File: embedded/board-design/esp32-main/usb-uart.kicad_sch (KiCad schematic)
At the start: 16 parts, among them J4 0473460001, U3 FT231XS

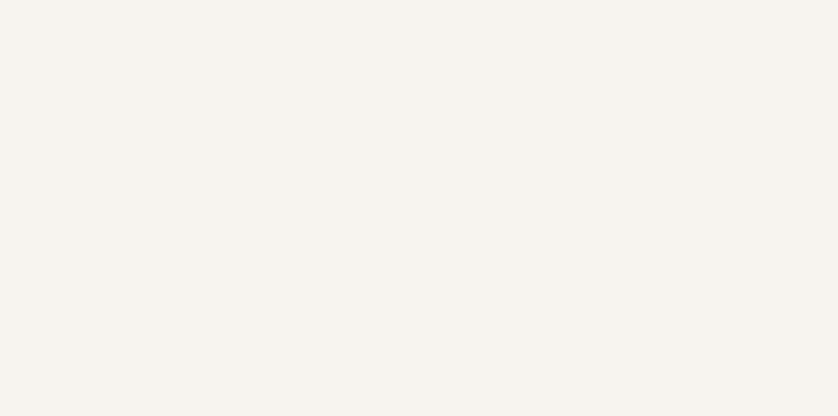
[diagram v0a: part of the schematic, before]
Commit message: [bike-embedded-app]
Signed-off-by: Nicolae-Andrei Vasile <vasilenicolaeandrei@gmail.com>
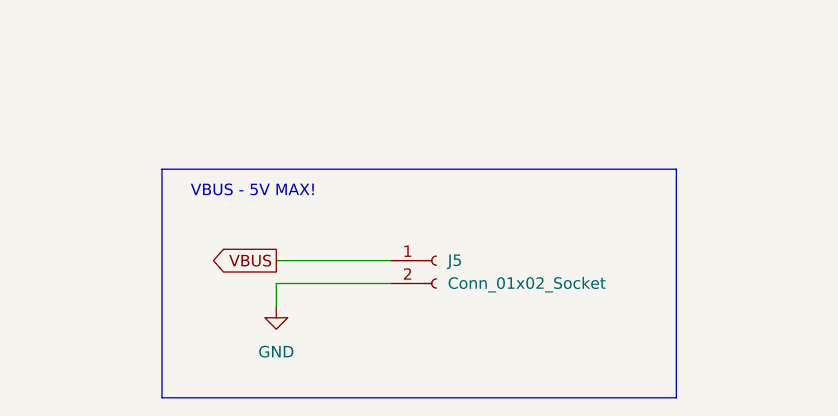
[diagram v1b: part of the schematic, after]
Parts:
- added J5: Conn_01x02_Socket, Connector_PinHeader_1.27mm:PinHeader_1x02_P1.27mm_Vertical, symbol Connector:Conn_01x02_Socket
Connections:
- net GND: now also J5.2 (Pin_2)
- net VBUS: now also J5.1 (Pin_1)
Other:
- note added: "VBUS - 5V MAX!"
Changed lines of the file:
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@@
 	(wire
 		(pts
+			(xy 127 176.53) (xy 139.7 176.53)
+		)
+		(stroke
+			(width 0)
+			(type default)
+		)
+	)
+	(wire
+		(pts
 			(xy 148.59 60.96) (xy 148.59 63.5)
 		)
@@
 	(wire
 		(pts
+			(xy 127 179.07) (xy 127 181.61)
+		)
+		(stroke
+			(width 0)
+			(type default)
+		)
+	)
+	(wire
+		(pts
 			(xy 118.11 86.36) (xy 147.32 86.36)
 		)
@@
 		)
 	)
+	(polyline
+		(pts
+			(xy 114.3 191.77) (xy 171.45 191.77)
+		)
+		(stroke
+			(width 0)
+			(type default)
+		)
+	)
 	(wire
 		(pts
@@
 		)
 	)
+	(polyline
+		(pts
+			(xy 171.45 166.37) (xy 114.3 166.37)
+		)
+		(stroke
+			(width 0)
+			(type default)
+		)
+	)
 	(wire
 		(pts
@@
 	(wire
 		(pts
+			(xy 139.7 179.07) (xy 127 179.07)
+		)
+		(stroke
+			(width 0)
+			(type default)
+		)
+	)
+	(wire
+		(pts
 			(xy 68.58 111.76) (xy 68.58 129.54)
 		)
@@
 		)
 	)
+	(polyline
+		(pts
+			(xy 171.45 191.77) (xy 171.45 166.37)
+		)
+		(stroke
+			(width 0)
+			(type default)
+		)
+	)
 	(wire
 		(pts
@@
 		)
 	)
+	(polyline
+		(pts
+			(xy 114.3 166.37) (xy 114.3 191.77)
+		)
+		(stroke
+			(width 0)
+			(type default)
+		)
+	)
 	(wire
 		(pts
@@
 		)
 	)
+	(text "VBUS - 5V MAX!"
+		(exclude_from_sim no)
+		(at 124.46 168.91 0)
+		(effects
+			(font
+				(size 1.27 1.27)
+			)
+		)
+	)
 	(label "D+"
 		(at 78.74 96.52 0)
@@
 	)
 	(global_label "VBUS"
+		(shape output)
+		(at 127 176.53 180)
+		(fields_autoplaced yes)
+		(effects
+			(font
+				(size 1.27 1.27)
+			)
+			(justify right)
+		)
+		(property "Intersheetrefs" "${INTERSHEET_REFS}"
+			(at 119.1162 176.53 0)
+			(effects
+				(font
+					(size 1.27 1.27)
+				)
+				(justify right)
+				(hide yes)
+			)
+		)
+	)
+	(global_label "VBUS"
 		(shape input)
 		(at 236.22 113.03 0)
@@
 	)
 	(symbol
+		(lib_id "Connector:Conn_01x02_Socket")
+		(at 144.78 176.53 0)
+		(unit 1)
+		(exclude_from_sim no)
+		(in_bom yes)
+		(on_board yes)
+		(dnp no)
+		(fields_autoplaced yes)
+		(property "Reference" "J5"
+			(at 146.05 176.5299 0)
+			(effects
+				(font
+					(size 1.27 1.27)
+				)
+				(justify left)
+			)
+		)
+		(property "Value" "Conn_01x02_Socket"
+			(at 146.05 179.0699 0)
+			(effects
+				(font
+					(size 1.27 1.27)
+				)
+				(justify left)
+			)
+		)
+		(property "Footprint" "Connector_PinHeader_1.27mm:PinHeader_1x02_P1.27mm_Vertical"
+			(at 144.78 176.53 0)
+			(effects
+				(font
+					(size 1.27 1.27)
+				)
+				(hide yes)
+			)
+		)
+		(property "Datasheet" "~"
+			(at 144.78 176.53 0)
+			(effects
+				(font
+					(size 1.27 1.27)
+				)
+				(hide yes)
+			)
+		)
+		(property "Description" "Generic connector, single row, 01x02, script generated"
+			(at 144.78 176.53 0)
+			(effects
+				(font
+					(size 1.27 1.27)
+				)
+				(hide yes)
+			)
+		)
+		(pin "1"
+		)
+		(pin "2"
+		)
+		(instances
+			(project "esp32-main"
+				(path "/6d02e045-d1b3-4320-a4f8-f5e2c734acd4/7d21a99c-c3fd-4678-bc5b-fcb8ce659019"
+					(reference "J5")
+					(unit 1)
+				)
+			)
+		)
+	)
+	(symbol
 		(lib_id "Device:R")
 		(at 194.31 114.3 90)
@@
 					(unit 1)
 				)
+			)
+		)
+	)
+	(symbol
+		(lib_id "power:GND")
+		(at 127 181.61 0)
+		(unit 1)
+		(exclude_from_sim no)
+		(in_bom yes)
+		(on_board yes)
+		(dnp no)
+		(fields_autoplaced yes)
+		(property "Reference" "#PWR015"
+			(at 127 187.96 0)
+			(effects
+				(font
+					(size 1.27 1.27)
+				)
+				(hide yes)
+			)
+		)
+		(property "Value" "GND"
+			(at 127 186.69 0)
+			(effects
+				(font
+					(size 1.27 1.27)
+				)
+			)
+		)
+		(property "Footprint" ""
+			(at 127 181.61 0)
+			(effects
+				(font
+					(size 1.27 1.27)
+				)
+				(hide yes)
+			)
+		)
+		(property "Datasheet" ""
+			(at 127 181.61 0)
+			(effects
+				(font
+					(size 1.27 1.27)
+				)
+				(hide yes)
+			)
+		)
+		(property "Description" "Power symbol creates a global label with name \"GND\" , ground"
+			(at 127 181.61 0)
+			(effects
+				(font
+					(size 1.27 1.27)
+				)
+				(hide yes)
+			)
+		)
+		(pin "1"
+		)
+		(instances
+			(project "esp32-main"
+				(path "/6d02e045-d1b3-4320-a4f8-f5e2c734acd4/7d21a99c-c3fd-4678-bc5b-fcb8ce659019"
+					(reference "#PWR015")
+					(unit 1)
+				)
